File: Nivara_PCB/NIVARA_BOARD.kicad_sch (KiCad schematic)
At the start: 3 parts, among them U1 ESP32-S3-WROOM-1

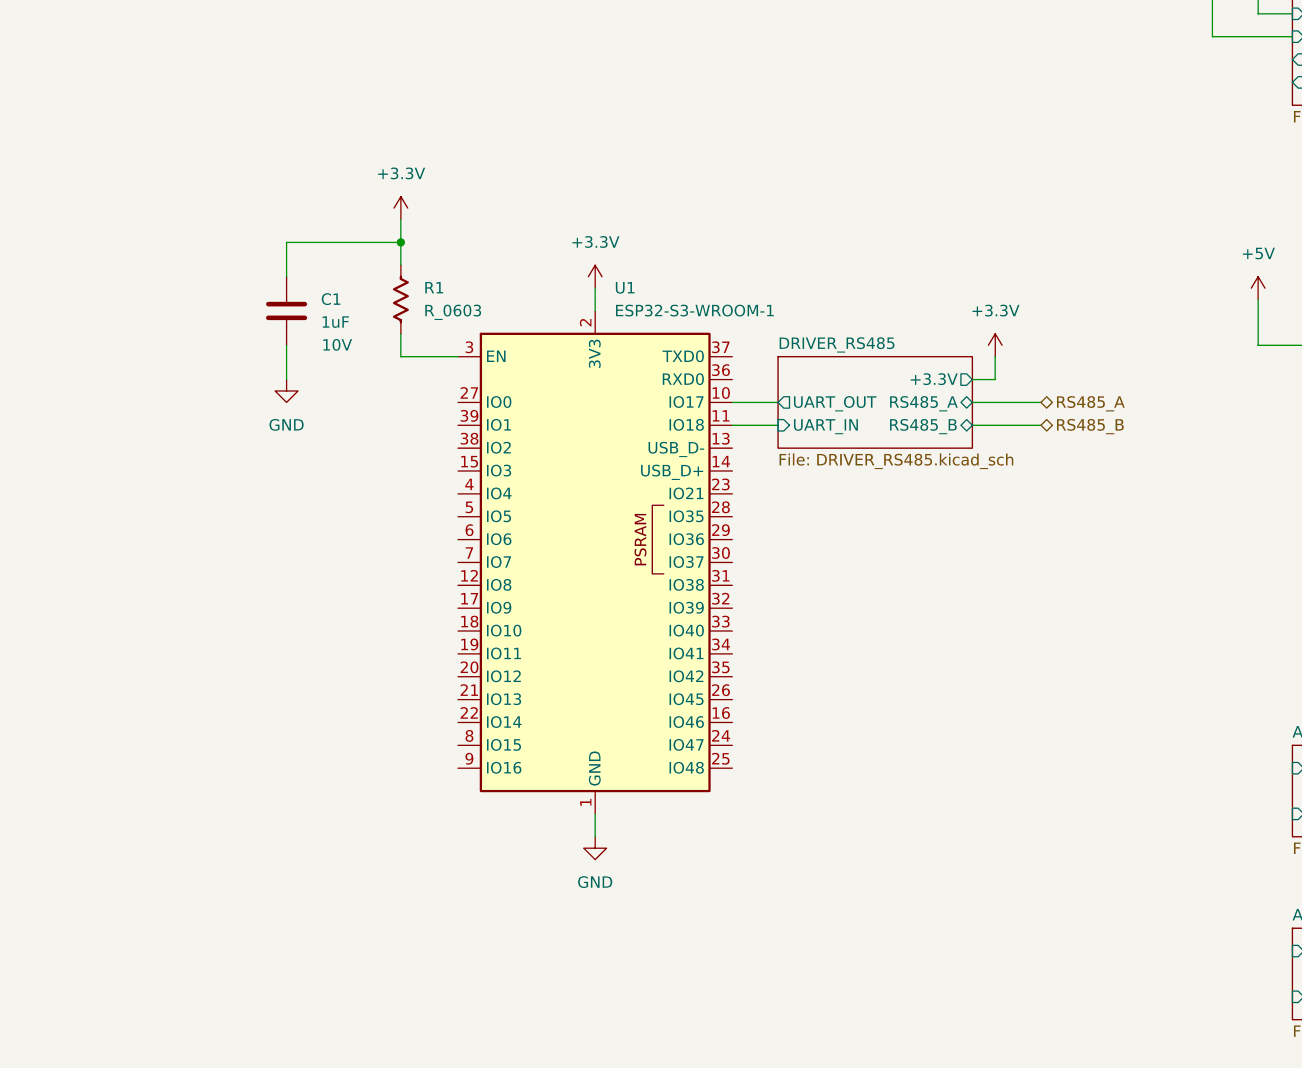
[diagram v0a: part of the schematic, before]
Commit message: Cambios en la power supply.
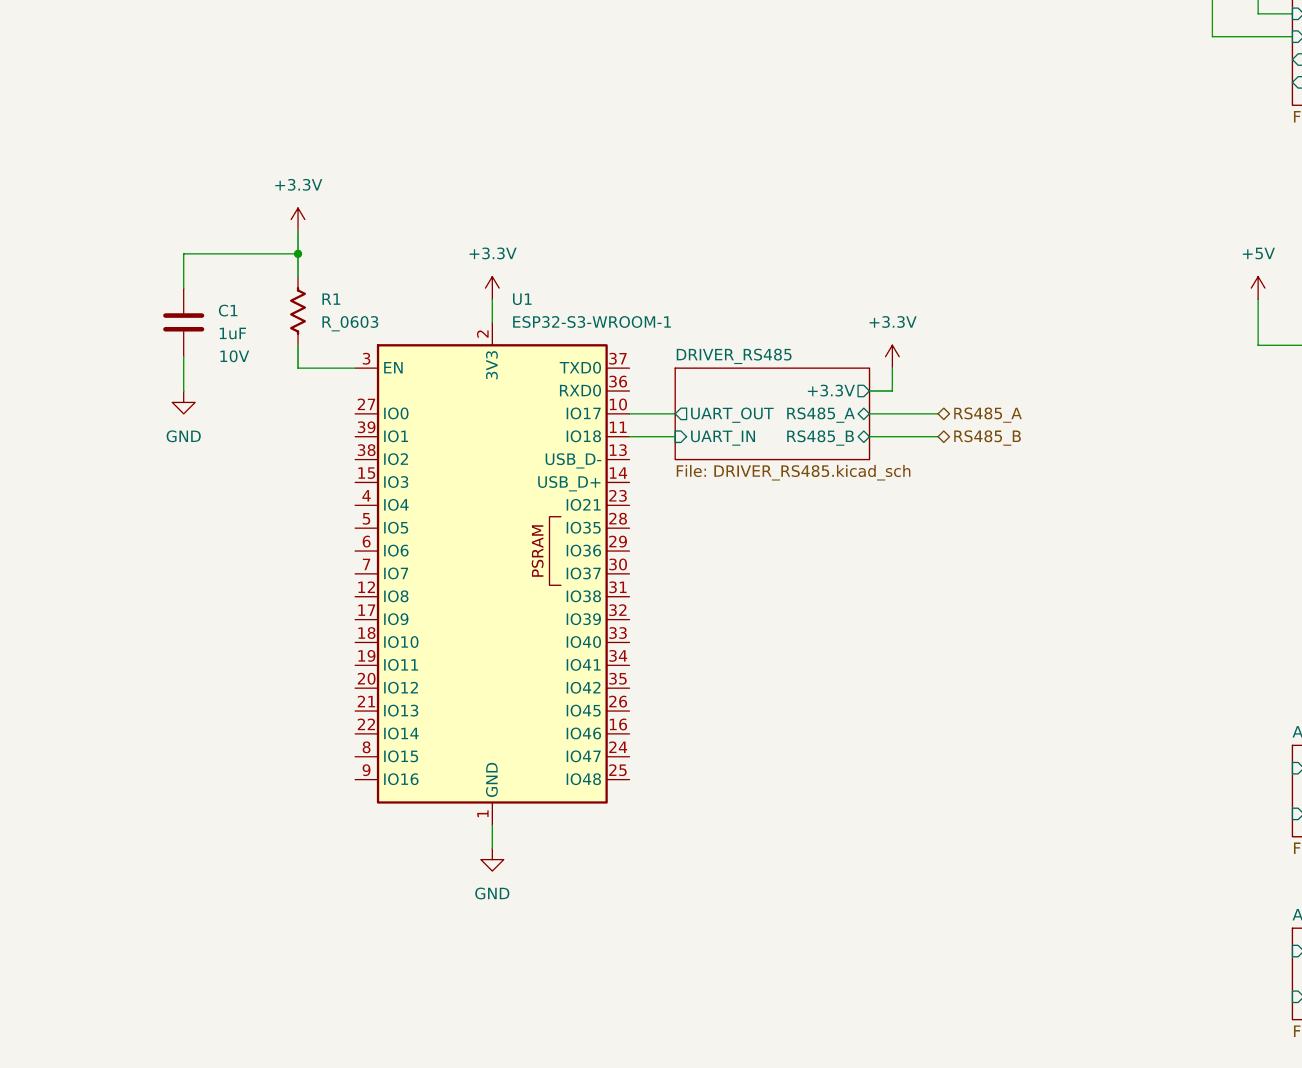
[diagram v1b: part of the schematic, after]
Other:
- moved on the sheet: C1, R1, U1
